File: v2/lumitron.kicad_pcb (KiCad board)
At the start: 2 copper layers, 40.6 x 78.7 mm, 11 parts

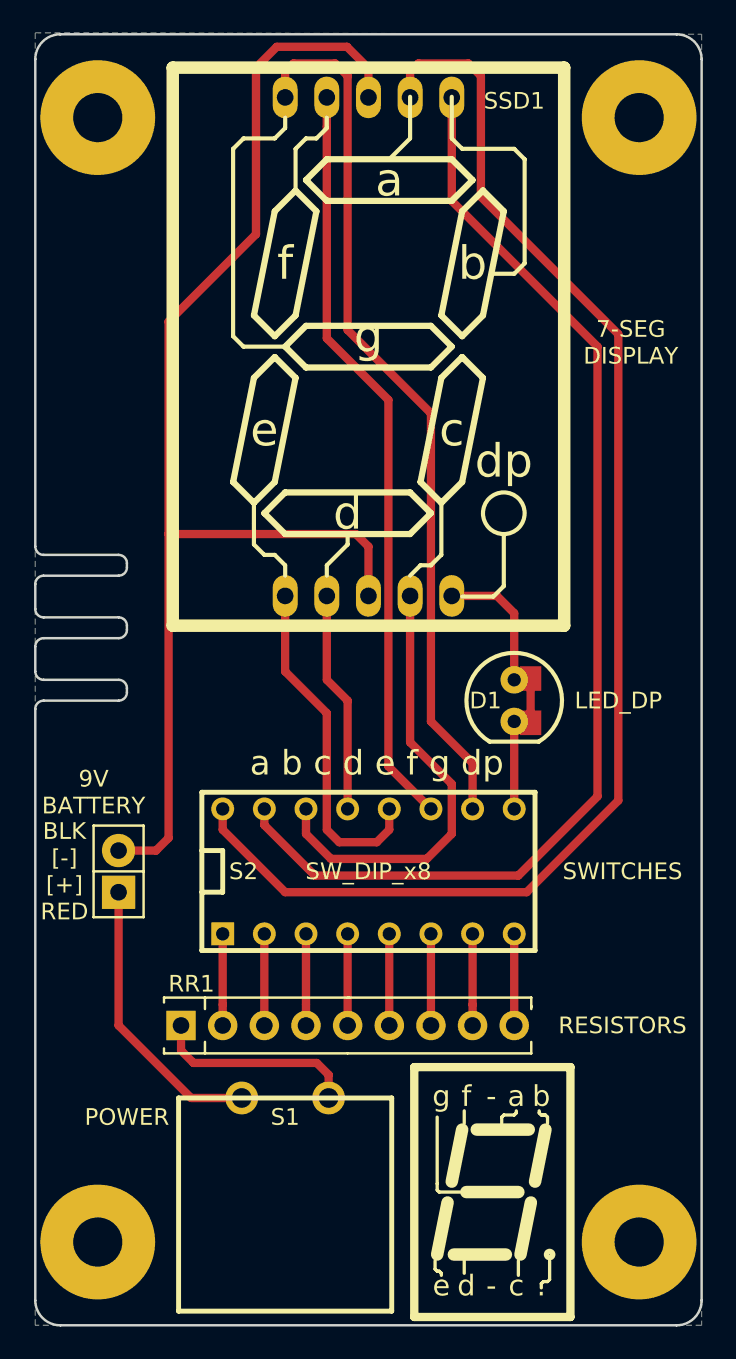
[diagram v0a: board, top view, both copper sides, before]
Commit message: track layout cleanup
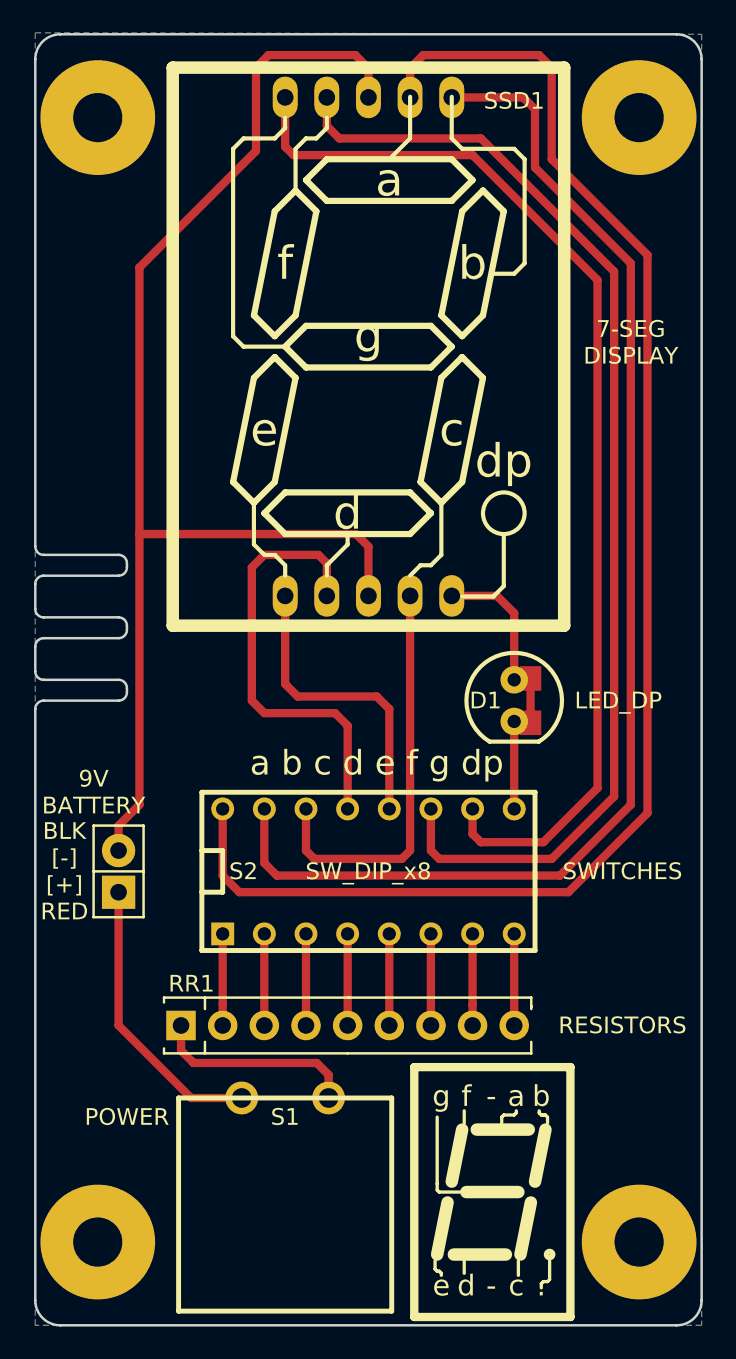
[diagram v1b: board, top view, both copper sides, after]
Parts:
- moved BT2 1.40 mm to (101.6, 96.5)
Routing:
- net /f: track 46.0 -> 70.5 mm
- net /g: track 53.8 -> 67.1 mm
- net /d: track 13.5 -> 26.8 mm
- net /a: track 83.4 -> 91.3 mm
- net /b: track 70.9 -> 78.0 mm
- net /e: track 21.0 -> 18.4 mm
- net /c: track 27.2 -> 24.8 mm
